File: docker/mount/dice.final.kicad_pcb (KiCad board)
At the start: 2 copper layers, 130 x 130 mm, 303 parts

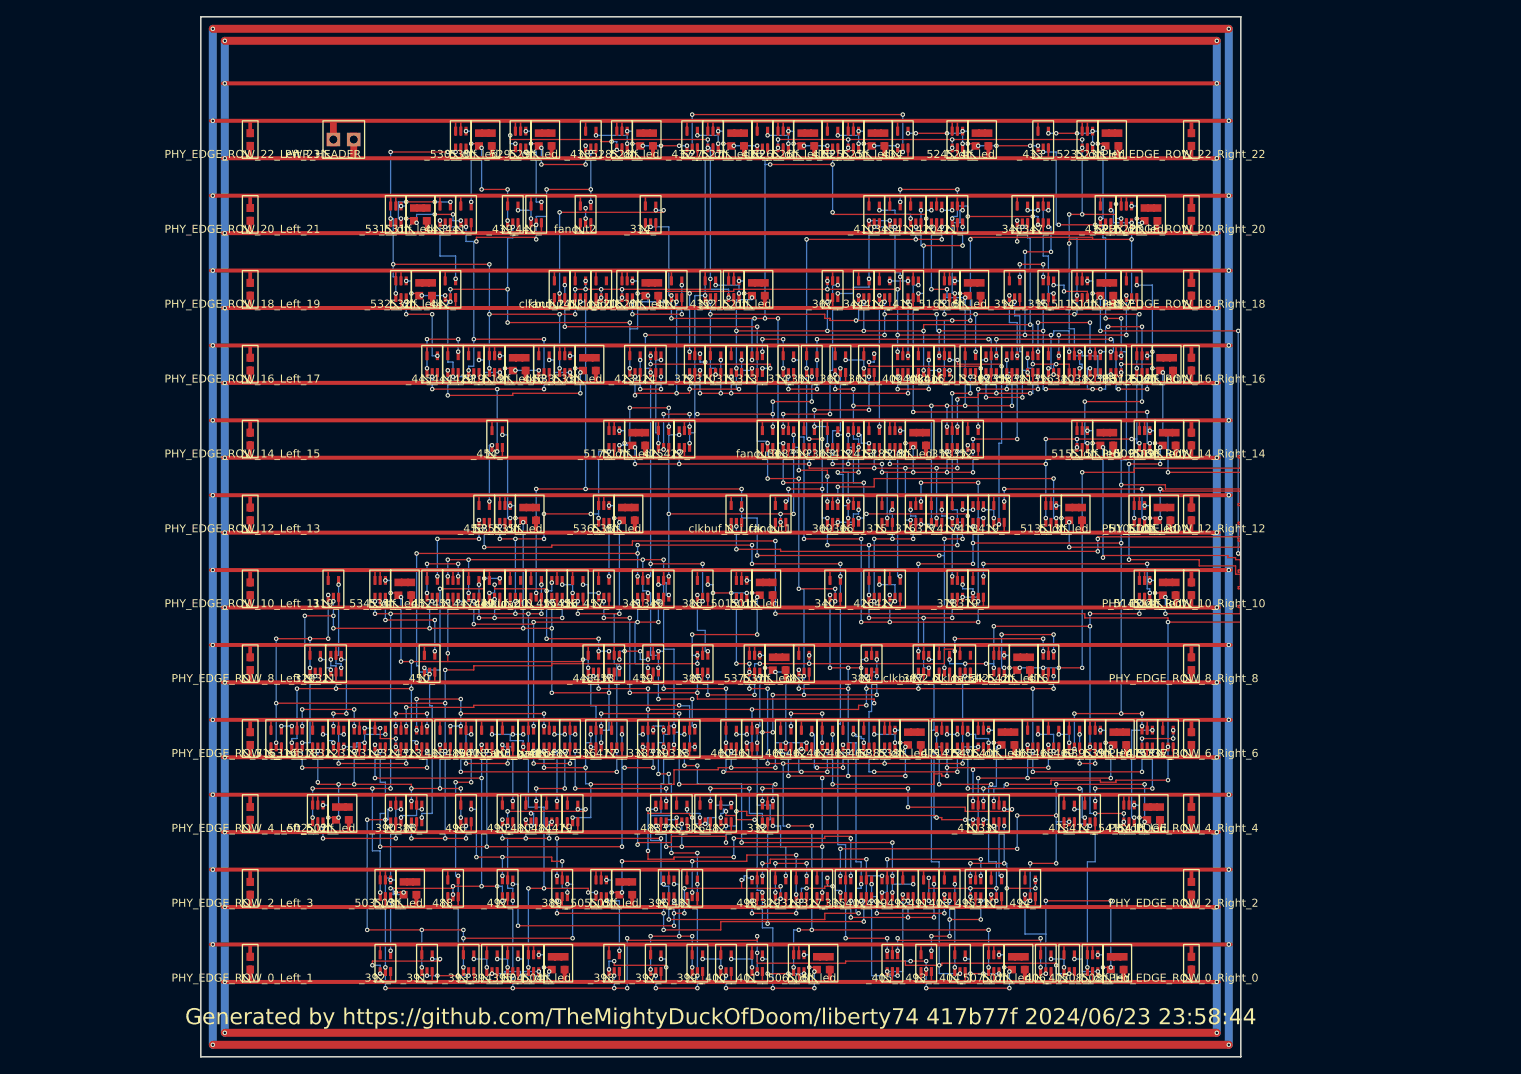
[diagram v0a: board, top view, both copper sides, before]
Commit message: Update example
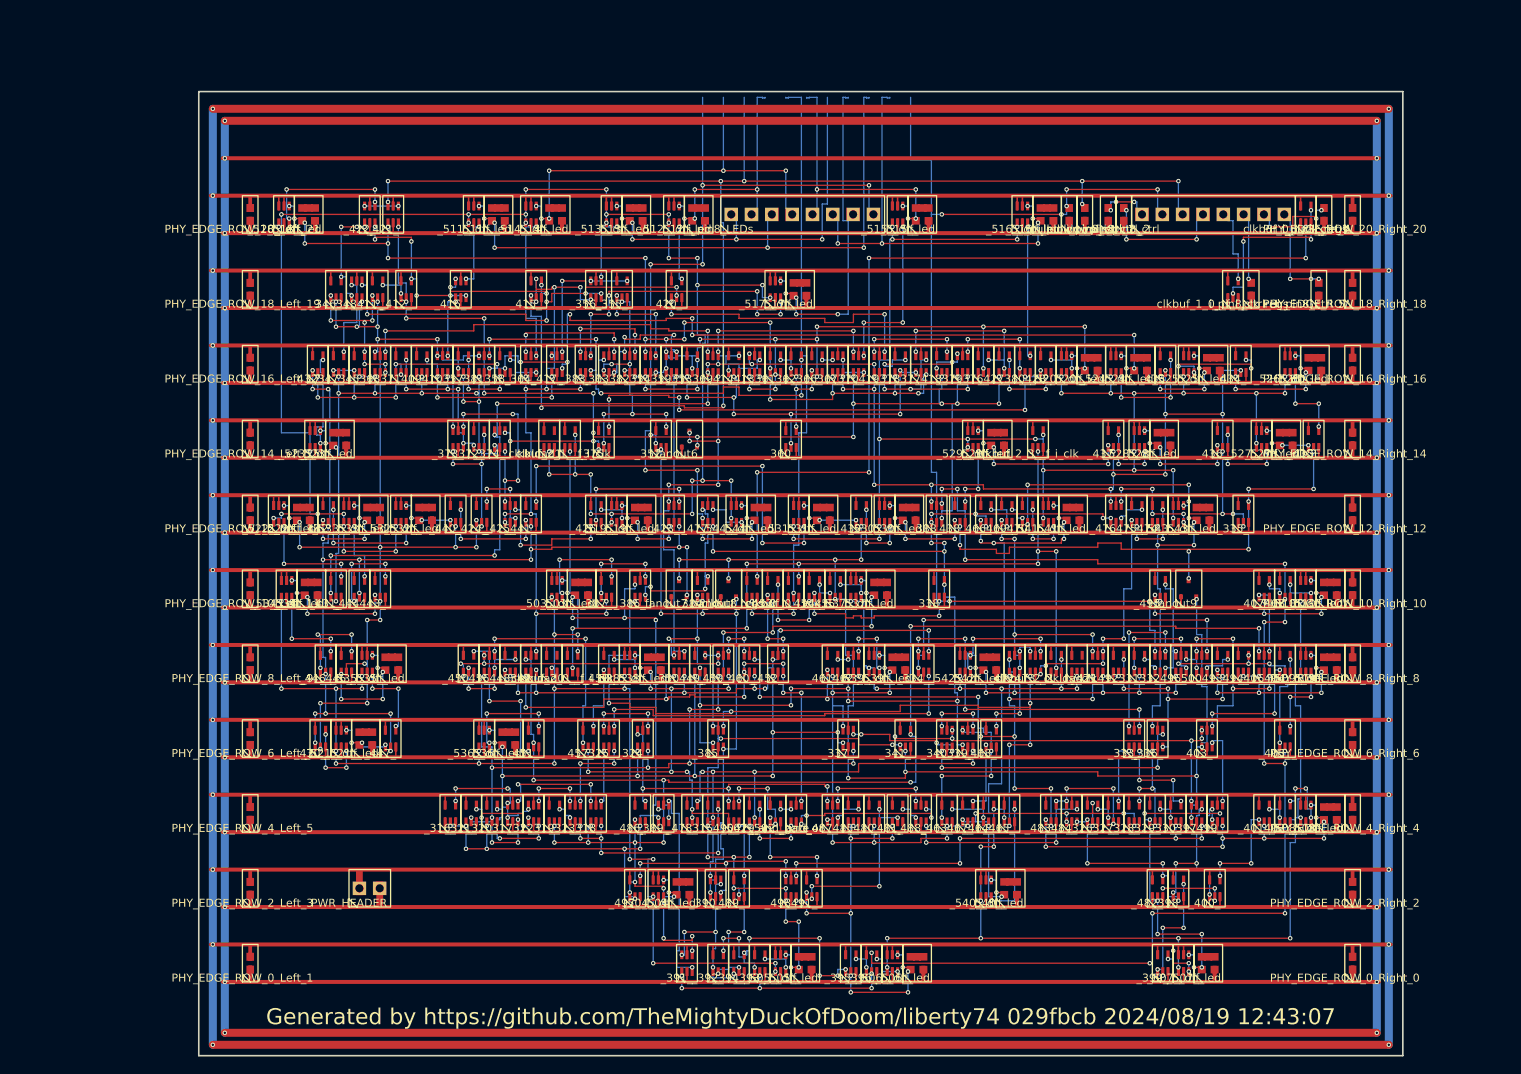
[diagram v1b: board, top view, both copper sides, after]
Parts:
- removed PHY_EDGE_ROW_22_Left_23, PHY_EDGE_ROW_22_Right_22: PWR_CAP, liberty74:PWR_CAP_N
- removed _314_: XOR2_74LVC1G86, liberty74:XOR2_74LVC1G86_N
- removed the _315_ at (8.12, -37.4)
- removed the _316_ at (10.7, -37.4)
- removed the _317_ at (18.5, -37.4)
- removed the _318_ at (13.3, -37.4)
- removed the _319_ at (15.3, -56.2)
- removed the _320_ at (13.0, -46.8)
- removed the _321_ at (15.6, -46.8)
- removed the _322_ at (15.9, -37.4)
- removed the _323_ at (26.3, -37.4)
- removed the _324_ at (23.7, -37.4)
- removed the _325_ at (58.8, -28.1)
- removed the _326_ at (61.8, -28.1)
- removed the _327_ at (76.4, -18.7)
- removed the _328_ at (73.8, -18.7)
- removed the _329_ at (71.2, -18.7)
- removed the _330_ at (98.2, -18.7)
- removed the _331_ at (98.5, -28.1)
- removed the _332_ at (69.5, -28.1)
- removed the _333_ at (59.8, -37.4)
- removed the _334_ at (54.9, -103.0)
- removed the _335_ at (79.3, -18.7)
- removed the _336_ at (48.1, -37.4)
- removed the _337_ at (119.6, -37.4)
- removed the _338_ at (54.6, -37.4)
- removed the _339_ at (57.2, -37.4)
- removed the _340_ at (78.0, -56.2)
- removed the _341_ at (54.0, -56.2)
- removed _344_, _351_: NAND2_74LVC1G00, liberty74:NAND2_74LVC1G00_N
- removed the _346_ at (101.4, -103.0)
- removed the _347_ at (104.0, -103.0)
- removed _349_: NAND3_74LVC1G10, liberty74:NAND3_74LVC1G10_N
- removed the _352_ at (95.2, -74.9)
- removed the _353_ at (100.1, -84.2)
- removed the _354_ at (100.4, -93.6)
- removed the _355_ at (104.7, -93.6)
- removed the _356_ at (105.3, -84.2)
- removed the _357_ at (115.0, -93.6)
- removed the _358_ at (92.6, -74.9)
- removed the _359_ at (74.8, -74.9)
- removed the _360_ at (78.7, -84.2)
- removed the _361_ at (82.2, -84.2)
- removed the _362_ at (97.5, -84.2)
- removed the _363_ at (113.1, -84.2)
- removed _365_, _429_, _500__and_gate: AND2_74LVC1G08, liberty74:AND2_74LVC1G08_N
- removed the _366_ at (80.3, -65.5)
- removed the _367_ at (77.7, -93.6)
- removed the _368_ at (72.2, -74.9)
- removed the _369_ at (77.7, -65.5)
- removed the _370_ at (63.0, -84.2)
- removed the _371_ at (65.7, -84.2)
- removed the _372_ at (60.5, -84.2)
- removed the _373_ at (68.2, -84.2)
- removed the _374_ at (72.2, -84.2)
- removed the _375_ at (84.5, -65.5)
- removed the _376_ at (88.1, -65.5)
- removed the _377_ at (90.7, -65.5)
- removed the _378_ at (93.3, -56.2)
- removed the _379_ at (95.9, -56.2)
- removed the _380_ at (107.9, -84.2)
- removed the _381_ at (102.7, -84.2)
- removed the _382_ at (110.5, -84.2)
- removed the _383_ at (74.1, -46.8)
- removed the _384_ at (82.5, -46.8)
- removed the _385_ at (61.4, -46.8)
- removed the _386_ at (61.4, -56.2)
- removed the _387_ at (89.0, -46.8)
- removed the _389_ at (43.9, -18.7)
- removed the _390_ at (23.1, -28.1)
- removed the _391_ at (27.0, -9.36)
- removed the _392_ at (21.8, -9.36)
- removed the _393_ at (32.2, -9.36)
- removed the _394_ at (35.1, -9.36)
- removed the _395_ at (37.7, -9.36)
- removed the _396_ at (57.2, -18.7)
- removed the _397_ at (55.6, -9.36)
- removed the _398_ at (50.4, -9.36)
- removed the _399_ at (60.8, -9.36)
- removed the _400_ at (64.3, -9.36)
- removed the _401_ at (68.2, -9.36)
- removed the _402_ at (81.9, -18.7)
- removed the _403_ at (92.3, -18.7)
- removed the _404_ at (93.6, -9.36)
- removed the _405_ at (85.2, -9.36)
- removed the _406_ at (104.3, -9.36)
- removed the _407_ at (107.2, -9.36)
- removed the _408_ at (89.0, -84.2)
- removed the _409_ at (86.5, -84.2)
- removed the _410_ at (82.9, -103.0)
- removed the _412_ at (80.3, -74.9)
- removed the _413_ at (82.9, -74.9)
- removed the _414_ at (84.2, -93.6)
- removed the _415_ at (87.8, -93.6)
- removed the _416_ at (91.7, -84.2)
- removed the _417_ at (93.3, -65.5)
- removed the _418_ at (95.9, -65.5)
- removed the _419_ at (98.5, -65.5)
- removed the _420_ at (90.7, -103.0)
- removed the _422_ at (59.1, -74.9)
- removed the _423_ at (53.0, -84.2)
- removed the _424_ at (55.6, -84.2)
- removed the _425_ at (56.5, -74.9)
- removed the _426_ at (82.9, -56.2)
- removed the _427_ at (85.5, -56.2)
- removed the _430_ at (58.2, -93.6)
- removed the _431_ at (62.4, -93.6)
- removed the _432_ at (111.8, -103.0)
- removed the _434_ at (86.5, -112.3)
- removed the _435_ at (77.7, -112.3)
- removed the _437_ at (60.1, -112.3)
- removed the _439_ at (37.7, -103.0)
- removed the _440_ at (40.6, -103.0)
- removed the _442_ at (29.9, -93.6)
- removed the _443_ at (29.2, -103.0)
- removed the _444_ at (30.2, -84.2)
- removed the _445_ at (27.6, -84.2)
- removed the _449_ at (35.4, -56.2)
- removed the _450_ at (27.3, -46.8)
- removed the _451_ at (30.2, -56.2)
- removed the _452_ at (27.6, -56.2)
- removed the _453_ at (34.1, -65.5)
- removed the _454_ at (35.8, -74.9)
- removed the _455_ at (43.2, -56.2)
- removed the _456_ at (45.8, -56.2)
- removed the _457_ at (49.1, -56.2)
- removed the _458_ at (50.4, -46.8)
- removed the _460_ at (65.0, -37.4)
- removed the _461_ at (67.6, -37.4)
- removed the _462_ at (74.4, -37.4)
- removed the _463_ at (79.6, -37.4)
- removed the _464_ at (82.2, -37.4)
- removed the _468_ at (105.3, -37.4)
- removed the _469_ at (107.9, -37.4)
- removed the _470_ at (95.9, -28.1)
- removed the _471_ at (91.3, -37.4)
- removed the _472_ at (93.9, -37.4)
- removed the _473_ at (107.2, -28.1)
- removed the _474_ at (109.8, -28.1)
- removed the _475_ at (117.0, -37.4)
- removed the _477_ at (50.7, -37.4)
- removed the _478_ at (34.5, -37.4)
- removed the _479_ at (45.2, -28.1)
- removed the _480_ at (40.0, -28.1)
- removed the _481_ at (60.1, -18.7)
- removed the _482_ at (64.3, -28.1)
- removed the _483_ at (56.2, -28.1)
- removed the _484_ at (42.6, -28.1)
- removed the _485_ at (29.2, -37.4)
- removed the _486_ at (42.2, -37.4)
- removed the _488_ at (30.2, -18.7)
- removed the _489_ at (31.9, -37.4)
- removed the _490_ at (37.0, -28.1)
- removed the _491_ at (89.7, -18.7)
- removed the _492_ at (87.1, -18.7)
- removed the _493_ at (89.4, -9.36)
- removed the _494_ at (102.4, -18.7)
- removed the _495_ at (95.5, -18.7)
- removed the _496_ at (31.9, -28.1)
- removed the _497_ at (37.0, -18.7)
- removed the _499_ at (84.5, -18.7)
- removed _500__and_or: AO21_74LVC1G0832, liberty74:AO21_74LVC1G0832_N
- removed _501__dff, _502__dff: DFF_74LVC1G175, liberty74:DFF_74LVC1G175_N
- removed _501__led, _502__led: Led_Res_0603, liberty74:Led_Res_0603_N
- removed fanout1, fanout2, fanout3, fanout4: BUF_74LVC1G125, liberty74:BUF_74LVC1G125_N
- added _315_: XOR2_74LVC1G86, liberty74:XOR2_74LVC1G86_N, F.Cu at (62.7, -28.1)
- added _316_: INV_74LVC1G04, liberty74:INV_74LVC1G04_N, F.Cu at (29.9, -28.1)
- added _317_: AND3_74LVC1G11, liberty74:AND3_74LVC1G11_N, F.Cu at (37.7, -28.1)
- added _318_: NAND3_74LVC1G10, liberty74:NAND3_74LVC1G10_N, F.Cu at (48.1, -28.1)
- added _319_: INV_74LVC1G04, liberty74:INV_74LVC1G04_N, F.Cu at (42.9, -28.1)
- added _320_: AND2_74LVC1G08, liberty74:AND2_74LVC1G08_N, F.Cu at (35.1, -28.1)
- added _321_: NOR2_74LVC1G02, liberty74:NOR2_74LVC1G02_N, F.Cu at (32.5, -28.1)
- added _322_: MUX2_74LVC1G157, liberty74:MUX2_74LVC1G157_N, F.Cu at (40.3, -28.1)
- added _323_: NAND3_74LVC1G10, liberty74:NAND3_74LVC1G10_N, F.Cu at (45.5, -28.1)
- added _324_: OR3_74LVC1G332, liberty74:OR3_74LVC1G332_N, F.Cu at (54.0, -37.4)
- added _325_: NAND3_74LVC1G10, liberty74:NAND3_74LVC1G10_N, F.Cu at (49.7, -37.4)
- added _326_: OR2_74LVC1G32, liberty74:OR2_74LVC1G32_N, F.Cu at (110.2, -28.1)
- added _327_: AND2_74LVC1G08, liberty74:AND2_74LVC1G08_N, F.Cu at (112.8, -28.1)
- added _328_: INV_74LVC1G04, liberty74:INV_74LVC1G04_N, F.Cu at (115.4, -28.1)
- added _329_: XOR2_74LVC1G86, liberty74:XOR2_74LVC1G86_N, F.Cu at (118.0, -28.1)
- added _330_: NOR2_74LVC1G02, liberty74:NOR2_74LVC1G02_N, F.Cu at (120.6, -28.1)
- added _331_: OR2_74LVC1G32, liberty74:OR2_74LVC1G32_N, F.Cu at (116.0, -46.8)
- added _332_: AO21_74LVC1G0832, liberty74:AO21_74LVC1G0832_N, F.Cu at (118.6, -46.8)
- added _333_: NOR3_74LVC1G27, liberty74:NOR3_74LVC1G27_N, F.Cu at (115.4, -37.4)
- added _334_: AND3_74LVC1G11, liberty74:AND3_74LVC1G11_N, F.Cu at (89.0, -46.8)
- added _335_: INV_74LVC1G04, liberty74:INV_74LVC1G04_N, F.Cu at (129.0, -65.5)
- added _336_: AND3_74LVC1G11, liberty74:AND3_74LVC1G11_N, F.Cu at (118.3, -37.4)
- added _337_: NOR3_74LVC1G27, liberty74:NOR3_74LVC1G27_N, F.Cu at (79.6, -37.4)
- added _338_: INV_74LVC1G04, liberty74:INV_74LVC1G04_N, F.Cu at (91.0, -56.2)
- added _339_: AND3_74LVC1G11, liberty74:AND3_74LVC1G11_N, F.Cu at (94.6, -37.4)
- added _340_: NAND3_74LVC1G10, liberty74:NAND3_74LVC1G10_N, F.Cu at (92.0, -37.4)
- added _341_: AND2_74LVC1G08, liberty74:AND2_74LVC1G08_N, F.Cu at (86.8, -37.4)
- added _342_: AND3_74LVC1G11, liberty74:AND3_74LVC1G11_N, F.Cu at (40.0, -46.8)
- added _346_: NAND2_74LVC1G00, liberty74:NAND2_74LVC1G00_N, F.Cu at (15.6, -93.6)
- added _347_: OR2_74LVC1G32, liberty74:OR2_74LVC1G32_N, F.Cu at (15.9, -84.2)
- added _348_: MUX2_74LVC1G157, liberty74:MUX2_74LVC1G157_N, F.Cu at (18.2, -93.6)
- added _350_: NAND3_74LVC1G10, liberty74:NAND3_74LVC1G10_N, F.Cu at (58.5, -46.8)
- added _352_: NAND2_74LVC1G00, liberty74:NAND2_74LVC1G00_N, F.Cu at (56.2, -74.9)
- added _353_: NOR2_74LVC1G02, liberty74:NOR2_74LVC1G02_N, F.Cu at (60.1, -84.2)
- added _354_: MUX2_74LVC1G157, liberty74:MUX2_74LVC1G157_N, F.Cu at (54.9, -84.2)
- added _355_: NOR2_74LVC1G02, liberty74:NOR2_74LVC1G02_N, F.Cu at (51.4, -93.6)
- added _356_: AO21_74LVC1G0832, liberty74:AO21_74LVC1G0832_N, F.Cu at (48.1, -93.6)
- added _357_: XOR2_74LVC1G86, liberty74:XOR2_74LVC1G86_N, F.Cu at (31.5, -84.2)
- added _358_: OR2_74LVC1G32, liberty74:OR2_74LVC1G32_N, F.Cu at (36.7, -84.2)
- added _359_: AND3_74LVC1G11, liberty74:AND3_74LVC1G11_N, F.Cu at (57.5, -84.2)
- added _360_: INV_74LVC1G04, liberty74:INV_74LVC1G04_N, F.Cu at (72.5, -74.9)
- added _361_: XOR2_74LVC1G86, liberty74:XOR2_74LVC1G86_N, F.Cu at (70.5, -84.2)
- added _362_: AND2_74LVC1G08, liberty74:AND2_74LVC1G08_N, F.Cu at (73.1, -84.2)
- added _363_: NOR3_74LVC1G27, liberty74:NOR3_74LVC1G27_N, F.Cu at (49.7, -84.2)
- added _364_: AO21_74LVC1G0832, liberty74:AO21_74LVC1G0832_N, F.Cu at (40.0, -84.2)
- added _366_: AND2_74LVC1G08, liberty74:AND2_74LVC1G08_N, F.Cu at (75.7, -84.2)
- added _367_: NOR3_74LVC1G27, liberty74:NOR3_74LVC1G27_N, F.Cu at (78.3, -84.2)
- added _368_: MUX2_74LVC1G157, liberty74:MUX2_74LVC1G157_N, F.Cu at (21.1, -84.2)
- added _369_: NOR3_74LVC1G27, liberty74:NOR3_74LVC1G27_N, F.Cu at (62.7, -84.2)
- added _370_: AO21_74LVC1G0832, liberty74:AO21_74LVC1G0832_N, F.Cu at (80.9, -84.2)
- added _371_: INV_74LVC1G04, liberty74:INV_74LVC1G04_N, F.Cu at (23.7, -84.2)
- added _372_: OR2_74LVC1G32, liberty74:OR2_74LVC1G32_N, F.Cu at (33.5, -74.9)
- added _373_: NAND3_74LVC1G10, liberty74:NAND3_74LVC1G10_N, F.Cu at (30.9, -74.9)
- added _374_: AO21_74LVC1G0832, liberty74:AO21_74LVC1G0832_N, F.Cu at (36.1, -74.9)
- added _375_: AND2_74LVC1G08, liberty74:AND2_74LVC1G08_N, F.Cu at (49.1, -74.9)
- added _376_: INV_74LVC1G04, liberty74:INV_74LVC1G04_N, F.Cu at (96.5, -84.2)
- added _377_: AO21_74LVC1G0832, liberty74:AO21_74LVC1G0832_N, F.Cu at (88.7, -84.2)
- added _378_: OR2_74LVC1G32, liberty74:OR2_74LVC1G32_N, F.Cu at (86.1, -84.2)
- added _379_: AND3_74LVC1G11, liberty74:AND3_74LVC1G11_N, F.Cu at (93.9, -84.2)
- added _380_: NOR2_74LVC1G02, liberty74:NOR2_74LVC1G02_N, F.Cu at (101.7, -84.2)
- added _381_: OR3_74LVC1G332, liberty74:OR3_74LVC1G332_N, F.Cu at (34.1, -84.2)
- added _382_: NOR3_74LVC1G27, liberty74:NOR3_74LVC1G27_N, F.Cu at (52.3, -84.2)
- added _383_: AO21_74LVC1G0832, liberty74:AO21_74LVC1G0832_N, F.Cu at (46.8, -84.2)
- added _384_: NAND2_74LVC1G00, liberty74:NAND2_74LVC1G00_N, F.Cu at (61.4, -56.2)
- added _385_: AND3_74LVC1G11, liberty74:AND3_74LVC1G11_N, F.Cu at (63.4, -37.4)
- added _386_: MUX2_74LVC1G157, liberty74:MUX2_74LVC1G157_N, F.Cu at (53.6, -56.2)
- added _387_: NOR2_74LVC1G02, liberty74:NOR2_74LVC1G02_N, F.Cu at (49.4, -56.2)
- added _389_: AO21_74LVC1G0832, liberty74:AO21_74LVC1G0832_N, F.Cu at (56.5, -28.1)
- added _390_: NAND3_74LVC1G10, liberty74:NAND3_74LVC1G10_N, F.Cu at (63.0, -18.7)
- added _391_: AND3_74LVC1G11, liberty74:AND3_74LVC1G11_N, F.Cu at (59.5, -9.36)
- added _392_: XOR2_74LVC1G86, liberty74:XOR2_74LVC1G86_N, F.Cu at (63.4, -9.36)
- added _393_: AND2_74LVC1G08, liberty74:AND2_74LVC1G08_N, F.Cu at (68.6, -9.36)
- added _394_: NOR2_74LVC1G02, liberty74:NOR2_74LVC1G02_N, F.Cu at (66.0, -9.36)
- added _395_: XOR2_74LVC1G86, liberty74:XOR2_74LVC1G86_N, F.Cu at (80.0, -9.36)
- added _396_: AND2_74LVC1G08, liberty74:AND2_74LVC1G08_N, F.Cu at (82.5, -9.36)
- added _397_: NAND3_74LVC1G10, liberty74:NAND3_74LVC1G10_N, F.Cu at (123.2, -28.1)
- added _398_: XOR2_74LVC1G86, liberty74:XOR2_74LVC1G86_N, F.Cu at (120.9, -18.7)
- added _399_: AND2_74LVC1G08, liberty74:AND2_74LVC1G08_N, F.Cu at (119.0, -9.36)
- added _400_: NOR2_74LVC1G02, liberty74:NOR2_74LVC1G02_N, F.Cu at (125.5, -18.7)
- added _401_: XOR2_74LVC1G86, liberty74:XOR2_74LVC1G86_N, F.Cu at (131.6, -28.1)
- added _402_: AND2_74LVC1G08, liberty74:AND2_74LVC1G08_N, F.Cu at (134.2, -28.1)
- added _403_: NAND3_74LVC1G10, liberty74:NAND3_74LVC1G10_N, F.Cu at (124.5, -37.4)
- added _404_: XOR2_74LVC1G86, liberty74:XOR2_74LVC1G86_N, F.Cu at (134.2, -46.8)
- added _405_: AND2_74LVC1G08, liberty74:AND2_74LVC1G08_N, F.Cu at (134.2, -37.4)
- added _406_: AND3_74LVC1G11, liberty74:AND3_74LVC1G11_N, F.Cu at (131.6, -46.8)
- added _407_: XOR2_74LVC1G86, liberty74:XOR2_74LVC1G86_N, F.Cu at (131.6, -56.2)
- added _408_: AND2_74LVC1G08, liberty74:AND2_74LVC1G08_N, F.Cu at (134.2, -56.2)
- added _409_: INV_74LVC1G04, liberty74:INV_74LVC1G04_N, F.Cu at (26.3, -84.2)
- added _410_: NAND3_74LVC1G10, liberty74:NAND3_74LVC1G10_N, F.Cu at (28.9, -84.2)
- added _412_: NOR2_74LVC1G02, liberty74:NOR2_74LVC1G02_N, F.Cu at (24.4, -93.6)
- added _413_: NOR3_74LVC1G27, liberty74:NOR3_74LVC1G27_N, F.Cu at (67.9, -84.2)
- added _414_: AND2_74LVC1G08, liberty74:AND2_74LVC1G08_N, F.Cu at (65.3, -84.2)
- added _415_: NOR2_74LVC1G02, liberty74:NOR2_74LVC1G02_N, F.Cu at (40.6, -93.6)
- added _416_: AO21_74LVC1G0832, liberty74:AO21_74LVC1G0832_N, F.Cu at (31.2, -93.6)
- added _417_: NAND3_74LVC1G10, liberty74:NAND3_74LVC1G10_N, F.Cu at (43.2, -84.2)
- added _418_: NAND2_74LVC1G00, liberty74:NAND2_74LVC1G00_N, F.Cu at (91.3, -84.2)
- added _419_: OR3_74LVC1G332, liberty74:OR3_74LVC1G332_N, F.Cu at (83.5, -84.2)
- added _420_: AND2_74LVC1G08, liberty74:AND2_74LVC1G08_N, F.Cu at (58.2, -93.6)
- added _422_: AO21_74LVC1G0832, liberty74:AO21_74LVC1G0832_N, F.Cu at (19.8, -103.0)
- added _423_: AND3_74LVC1G11, liberty74:AND3_74LVC1G11_N, F.Cu at (57.9, -65.5)
- added _424_: OR2_74LVC1G32, liberty74:OR2_74LVC1G32_N, F.Cu at (33.8, -65.5)
- added _425_: AND3_74LVC1G11, liberty74:AND3_74LVC1G11_N, F.Cu at (37.4, -65.5)
- added _426_: OR2_74LVC1G32, liberty74:OR2_74LVC1G32_N, F.Cu at (48.1, -65.5)
- added _427_: AND2_74LVC1G08, liberty74:AND2_74LVC1G08_N, F.Cu at (99.1, -84.2)
- added _428_: NOR2_74LVC1G02, liberty74:NOR2_74LVC1G02_N, F.Cu at (104.3, -84.2)
- added _430_: AND2_74LVC1G08, liberty74:AND2_74LVC1G08_N, F.Cu at (13.7, -37.4)
- added _431_: OR2_74LVC1G32, liberty74:OR2_74LVC1G32_N, F.Cu at (15.6, -56.2)
- added _432_: AND2_74LVC1G08, liberty74:AND2_74LVC1G08_N, F.Cu at (13.3, -84.2)
- added _434_: OR2_74LVC1G32, liberty74:OR2_74LVC1G32_N, F.Cu at (128.7, -84.2)
- added _435_: AND2_74LVC1G08, liberty74:AND2_74LVC1G08_N, F.Cu at (137.8, -74.9)
- added _437_: OR2_74LVC1G32, liberty74:OR2_74LVC1G32_N, F.Cu at (112.8, -74.9)
- added _439_: AND2_74LVC1G08, liberty74:AND2_74LVC1G08_N, F.Cu at (81.2, -65.5)
- added _440_: XOR2_74LVC1G86, liberty74:XOR2_74LVC1G86_N, F.Cu at (30.6, -65.5)
- added _442_: AND2_74LVC1G08, liberty74:AND2_74LVC1G08_N, F.Cu at (14.6, -65.5)
- added _443_: XOR2_74LVC1G86, liberty74:XOR2_74LVC1G86_N, F.Cu at (21.1, -56.2)
- added _444_: AND2_74LVC1G08, liberty74:AND2_74LVC1G08_N, F.Cu at (18.5, -56.2)
- added _445_: XOR2_74LVC1G86, liberty74:XOR2_74LVC1G86_N, F.Cu at (16.9, -46.8)
- added _449_: AND2_74LVC1G08, liberty74:AND2_74LVC1G08_N, F.Cu at (61.1, -46.8)
- added _450_: XOR2_74LVC1G86, liberty74:XOR2_74LVC1G86_N, F.Cu at (32.2, -46.8)
- added _451_: AND2_74LVC1G08, liberty74:AND2_74LVC1G08_N, F.Cu at (40.3, -37.4)
- added _452_: AND3_74LVC1G11, liberty74:AND3_74LVC1G11_N, F.Cu at (70.8, -46.8)
- added _453_: XOR2_74LVC1G86, liberty74:XOR2_74LVC1G86_N, F.Cu at (70.2, -56.2)
- added _454_: OR2_74LVC1G32, liberty74:OR2_74LVC1G32_N, F.Cu at (75.4, -56.2)
- added _455_: AND2_74LVC1G08, liberty74:AND2_74LVC1G08_N, F.Cu at (78.0, -56.2)
- added _456_: AND3_74LVC1G11, liberty74:AND3_74LVC1G11_N, F.Cu at (34.8, -46.8)
- added _457_: XOR2_74LVC1G86, liberty74:XOR2_74LVC1G86_N, F.Cu at (47.1, -37.4)
- added _458_: AND2_74LVC1G08, liberty74:AND2_74LVC1G08_N, F.Cu at (49.7, -46.8)
- added _460_: AND3_74LVC1G11, liberty74:AND3_74LVC1G11_N, F.Cu at (67.3, -46.8)
- added _461_: XOR2_74LVC1G86, liberty74:XOR2_74LVC1G86_N, F.Cu at (77.7, -46.8)
- added _462_: AND3_74LVC1G11, liberty74:AND3_74LVC1G11_N, F.Cu at (80.3, -46.8)
- added _463_: AND2_74LVC1G08, liberty74:AND2_74LVC1G08_N, F.Cu at (92.0, -28.1)
- added _464_: XOR2_74LVC1G86, liberty74:XOR2_74LVC1G86_N, F.Cu at (97.2, -28.1)
- added _468_: AND2_74LVC1G08, liberty74:AND2_74LVC1G08_N, F.Cu at (97.5, -37.4)
- added _469_: XOR2_74LVC1G86, liberty74:XOR2_74LVC1G86_N, F.Cu at (99.5, -65.5)
- added _470_: OR2_74LVC1G32, liberty74:OR2_74LVC1G32_N, F.Cu at (102.0, -65.5)
- added _471_: NAND3_74LVC1G10, liberty74:NAND3_74LVC1G10_N, F.Cu at (110.8, -46.8)
- added _472_: AO21_74LVC1G0832, liberty74:AO21_74LVC1G0832_N, F.Cu at (100.4, -46.8)
- added _473_: AND3_74LVC1G11, liberty74:AND3_74LVC1G11_N, F.Cu at (103.0, -46.8)
- added _474_: INV_74LVC1G04, liberty74:INV_74LVC1G04_N, F.Cu at (118.3, -65.5)
- added _475_: XOR2_74LVC1G86, liberty74:XOR2_74LVC1G86_N, F.Cu at (115.7, -65.5)
- added _477_: AO21_74LVC1G0832, liberty74:AO21_74LVC1G0832_N, F.Cu at (62.1, -65.5)
- added _478_: INV_74LVC1G04, liberty74:INV_74LVC1G04_N, F.Cu at (60.1, -28.1)
- added _479_: AND2_74LVC1G08, liberty74:AND2_74LVC1G08_N, F.Cu at (67.9, -28.1)
- added _480_: INV_74LVC1G04, liberty74:INV_74LVC1G04_N, F.Cu at (82.9, -28.1)
- added _481_: AND2_74LVC1G08, liberty74:AND2_74LVC1G08_N, F.Cu at (85.8, -28.1)
- added _482_: INV_74LVC1G04, liberty74:INV_74LVC1G04_N, F.Cu at (118.3, -18.7)
- added _483_: XOR2_74LVC1G86, liberty74:XOR2_74LVC1G86_N, F.Cu at (105.0, -28.1)
- added _484_: AO21_74LVC1G0832, liberty74:AO21_74LVC1G0832_N, F.Cu at (107.6, -28.1)
- added _485_: INV_74LVC1G04, liberty74:INV_74LVC1G04_N, F.Cu at (80.3, -28.1)
- added _486_: NAND2_74LVC1G00, liberty74:NAND2_74LVC1G00_N, F.Cu at (53.6, -28.1)
- added _488_: AO21_74LVC1G0832, liberty74:AO21_74LVC1G0832_N, F.Cu at (88.7, -28.1)
- added _489_: INV_74LVC1G04, liberty74:INV_74LVC1G04_N, F.Cu at (66.0, -18.7)
- added _490_: AO21_74LVC1G0832, liberty74:AO21_74LVC1G0832_N, F.Cu at (65.3, -28.1)
- added _491_: XOR2_74LVC1G86, liberty74:XOR2_74LVC1G86_N, F.Cu at (75.1, -18.7)
- added _492_: INV_74LVC1G04, liberty74:INV_74LVC1G04_N, F.Cu at (113.4, -46.8)
- added _493_: XOR2_74LVC1G86, liberty74:XOR2_74LVC1G86_N, F.Cu at (126.4, -46.8)
- added _494_: INV_74LVC1G04, liberty74:INV_74LVC1G04_N, F.Cu at (129.0, -46.8)
- added _495_: XOR2_74LVC1G86, liberty74:XOR2_74LVC1G86_N, F.Cu at (118.6, -56.2)
- added _496_: AO21_74LVC1G0832, liberty74:AO21_74LVC1G0832_N, F.Cu at (121.2, -46.8)
- added _497_: AND2_74LVC1G08, liberty74:AND2_74LVC1G08_N, F.Cu at (53.0, -18.7)
- added _499_: AND3_74LVC1G11, liberty74:AND3_74LVC1G11_N, F.Cu at (125.8, -28.1)
- added _500_: MUX2_74LVC1G157, liberty74:MUX2_74LVC1G157_N, F.Cu at (123.8, -46.8)
- added _502__and_gate: AND2_74LVC1G08, liberty74:AND2_74LVC1G08_N, F.Cu at (70.5, -28.1)
- added _502__and_or: AO21_74LVC1G0832, liberty74:AO21_74LVC1G0832_N, F.Cu at (73.1, -28.1)
- added _543__dff: DFF_74LVC1G175, liberty74:DFF_74LVC1G175_N, F.Cu at (120.9, -65.5)
- added _543__led: Led_Res_0603, liberty74:Led_Res_0603_N, F.Cu at (123.5, -65.5)
- added _544__dff: DFF_74LVC1G175, liberty74:DFF_74LVC1G175_N, F.Cu at (65.7, -65.5)
- added _544__led: Led_Res_0603, liberty74:Led_Res_0603_N, F.Cu at (68.2, -65.5)
- added clkbuf_0_i_clk_regs: BUF_74LVC1G125, liberty74:BUF_74LVC1G125_N, F.Cu at (136.8, -103.0)
- added clkbuf_1_0__f_i_clk_regs: BUF_74LVC1G125, liberty74:BUF_74LVC1G125_N, F.Cu at (127.7, -93.6)
- added clkbuf_regs_0_: BUF_74LVC1G125, liberty74:BUF_74LVC1G125_N, F.Cu at (67.6, -56.2)
- added fanout6: DS9809PRSS3, liberty74:DS9809PRSS3_N, F.Cu at (59.5, -74.9)
- added fanout7: DS9809PRSS3, liberty74:DS9809PRSS3_N, F.Cu at (58.2, -56.2)
- added fanout8: DS9809PRSS3, liberty74:DS9809PRSS3_N, F.Cu at (64.3, -56.2)
- added fanout9: DS9809PRSS3, liberty74:DS9809PRSS3_N, F.Cu at (121.9, -56.2)
- added i_pin8_LEDs: PINOUT_8, liberty74:PINOUT_8_N, F.Cu at (65.0, -103.0)
- added i_pin8_ctrl: PINOUT_8, liberty74:PINOUT_8_N, F.Cu at (116.3, -103.0)
- added i_pin8_ctrl_1: TIE_LO, liberty74:TIE_LO_N, F.Cu at (112.5, -103.0)
- added i_pin8_ctrl_2: TIE_LO, liberty74:TIE_LO_N, F.Cu at (114.4, -103.0)
- added i_pin8_ctrl_3: TIE_LO, liberty74:TIE_LO_N, F.Cu at (130.3, -93.6)
- added i_pin8_ctrl_4: TIE_LO, liberty74:TIE_LO_N, F.Cu at (139.4, -103.0)
- added i_pin8_ctrl_5: TIE_LO, liberty74:TIE_LO_N, F.Cu at (138.8, -93.6)
- added i_pulldown_roll: PULLDOWN_R0603, liberty74:PULLDOWN_R0603_N, F.Cu at (107.6, -103.0)
- added i_pulldown_rst: PULLDOWN_R0603, liberty74:PULLDOWN_R0603_N, F.Cu at (109.5, -103.0)
- moved _522__dff 112.4 mm to (8.45, -65.5)
- moved _522__led 112.4 mm to (11.1, -65.5)
- moved _523__dff 103.5 mm to (13.0, -74.9)
- moved _523__led 103.5 mm to (15.6, -74.9)
- moved PWR_HEADER 93.7 mm to (18.5, -18.7)
- moved _514__dff 89.9 mm to (40.0, -103.0)
- moved _514__led 89.9 mm to (42.6, -103.0)
- moved _518__dff 81.4 mm to (9.10, -103.0)
- moved _518__led 81.4 mm to (11.7, -103.0)
- moved _527__dff 78.1 mm to (131.3, -74.9)
- moved _527__led 78.1 mm to (133.9, -74.9)
- moved _511__dff 76.6 mm to (32.8, -103.0)
- moved _511__led 76.6 mm to (35.4, -103.0)
- moved _388_ 75.0 mm to (90.7, -65.5)
- moved _528__dff 74.7 mm to (116.0, -74.9)
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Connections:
- net bcd[0] renamed segments\[5\]
- net bcd[1] renamed segments\[6\]
- net clkdiv[1] renamed lfsr\[14\]
- net clkdiv[2] renamed clkdiv\[0\]
- net counter[2] renamed counter\[0\]
- net counter[3] renamed counter\[1\]
- net counter[4] renamed counter\[2\]
- net counter[5] renamed counter\[3\]
- net counter[6] renamed counter\[4\]
- net counter[7] renamed counter\[5\]
- net lfsr[13] renamed lfsr\[11\]
- net lfsr[14] renamed lfsr\[12\]
- net lfsr[7] renamed lfsr\[5\]
- net segments[0] renamed segments\[2\]
- net segments[1] renamed counter\[7\]
- net segments[2] renamed counter\[6\]
- net segments[3] renamed segments\[1\]
- net segments[4] renamed segments\[0\]
- net segments[5] renamed segments\[3\]
- net segments[6] renamed segments\[4\]
- _345_ pad 1: _077_ -> lfsr\[3\]
- _345_ pad 2: lfsr[1] -> lfsr\[2\]
- _345_ pad 4: _078_ -> _077_
- _388_ pad 1: counter[0] -> _070_
- _388_ pad 3: _073_ -> net6
- _388_ pad 4: _115_ -> _114_
- _388_ pad 6: counter[1] -> RST
- _411_ pad 1: _130_ -> _077_
- _411_ pad 2: net1 -> lfsr\[1\]
- _411_ pad 4: _131_ -> _130_
- _421_ pad 1: _078_ -> bcd\[0\]
- _421_ pad 3: _131_ -> net6
- _421_ pad 4: _015_ -> _138_
- _421_ pad 6: _138_ -> RST
- _433_ pad 1: lfsr[5] -> lfsr\[4\]
- _433_ pad 4: _022_ -> _021_
- _436_ pad 1: lfsr[8] -> lfsr\[7\]
- _436_ pad 4: _025_ -> _024_
- _438_ pad 1: lfsr[10] -> lfsr\[9\]
- _438_ pad 2: net2 -> _067_
- _438_ pad 4: _027_ -> _026_
- _441_ pad 1: lfsr[12] -> _144_
- _441_ pad 2: net2 -> net7
- _441_ pad 4: _029_ -> _028_
- _446_ pad 1: lfsr[0] -> _146_
- _446_ pad 2: net2 -> net7
- _446_ pad 4: _032_ -> _031_
- _447_ pad 1: _066_ -> lfsr\[0\]
- _447_ pad 2: _183_ -> net7
- _447_ pad 4: _147_ -> _032_
- _448_ pad 1: clkdiv[0] -> _066_
- _448_ pad 2: _070_ -> _183_
- _448_ pad 4: _148_ -> _147_
- _459_ pad 1: _183_ -> clkdiv\[1\]
- _459_ pad 3: _066_ -> clkdiv\[2\]
- _459_ pad 4: _156_ -> _155_
- _459_ pad 6: _155_ -> _148_
- _465_ pad 1: clkdiv[5] -> _159_
- _465_ pad 2: _070_ -> _112_
- _465_ pad 4: _160_ -> _037_
- _466_ pad 1: clkdiv[4] -> clkdiv\[5\]
- _466_ pad 2: clkdiv[3] -> _070_
- _466_ pad 4: _161_ -> _160_
- _467_ pad 1: _161_ -> clkdiv\[4\]
- _467_ pad 2: _156_ -> clkdiv\[3\]
- _467_ pad 4: _162_ -> _161_
- _476_ pad 1: dp -> _070_
- _476_ pad 3: _070_ -> _167_
- _476_ pad 4: _041_ -> _040_
- _476_ pad 6: _111_ -> RST
- _487_ pad 1: _171_ -> clkdiv\[3\]
- _487_ pad 3: _174_ -> _175_
- _487_ pad 4: _178_ -> _177_
- _487_ pad 6: _177_ -> _176_
- _498_ pad 4: _045_ -> _044_
- _498_ pad 6: _044_ -> _043_
- _503__dff pad 3: _007_ -> _005_
- _504__dff pad 3: _008_ -> _006_
- _505__dff pad 3: _009_ -> _007_
- _506__dff pad 3: _010_ -> _008_
- _507__dff pad 3: _011_ -> _009_
- _508__dff pad 3: _012_ -> _010_
- _509__dff pad 1: clknet_2_3__leaf_i_clk -> clknet_2_2__leaf_i_clk
- _509__dff pad 3: _013_ -> _011_
- _510__dff pad 1: clknet_2_3__leaf_i_clk -> clknet_2_2__leaf_i_clk
- _510__dff pad 3: _014_ -> _012_
- _511__dff pad 1: clknet_2_3__leaf_i_clk -> clknet_2_1__leaf_i_clk
- _511__dff pad 3: _000_ -> _013_
- _512__dff pad 1: clknet_2_3__leaf_i_clk -> clknet_2_1__leaf_i_clk
- _512__dff pad 3: _001_ -> _014_
- _513__dff pad 1: clknet_2_3__leaf_i_clk -> clknet_2_1__leaf_i_clk
- _513__dff pad 3: _002_ -> _000_
- _514__dff pad 1: clknet_2_2__leaf_i_clk -> clknet_2_1__leaf_i_clk
- _514__dff pad 3: _003_ -> _001_
- _515__dff pad 3: _004_ -> _002_
- _516__dff pad 3: _015_ -> _003_
- _517__dff pad 1: clknet_2_0__leaf_i_clk -> clknet_2_1__leaf_i_clk
- _517__dff pad 3: _016_ -> _004_
- _518__dff pad 1: clknet_2_3__leaf_i_clk -> clknet_2_1__leaf_i_clk
- _518__dff pad 3: _017_ -> _015_
- _518__dff pad 4: bcd[2] -> bcd\[0\]
- _518__led pad 1: bcd[2] -> bcd\[0\]
- _519__dff pad 3: _018_ -> _016_
- _519__dff pad 4: lfsr[0] -> bcd\[1\]
- _519__led pad 1: lfsr[0] -> bcd\[1\]
- _520__dff pad 1: clknet_2_1__leaf_i_clk -> clknet_2_3__leaf_i_clk
- _520__dff pad 3: _019_ -> _017_
- _520__dff pad 4: lfsr[1] -> bcd\[2\]
- _520__led pad 1: lfsr[1] -> bcd\[2\]
- _521__dff pad 1: clknet_2_1__leaf_i_clk -> clknet_2_0__leaf_i_clk
- _521__dff pad 3: _020_ -> _018_
- _521__dff pad 4: lfsr[2] -> lfsr\[0\]
- _521__led pad 1: lfsr[2] -> lfsr\[0\]
- _522__dff pad 1: clknet_2_3__leaf_i_clk -> clknet_2_1__leaf_i_clk
- _522__dff pad 3: _021_ -> _019_
- _522__dff pad 4: lfsr[3] -> lfsr\[1\]
- _522__led pad 1: lfsr[3] -> lfsr\[1\]
- _523__dff pad 1: clknet_2_3__leaf_i_clk -> clknet_2_1__leaf_i_clk
- _523__dff pad 3: _022_ -> _020_
- _523__dff pad 4: lfsr[4] -> lfsr\[2\]
- _523__led pad 1: lfsr[4] -> lfsr\[2\]
- _524__dff pad 3: _023_ -> _021_
- _524__dff pad 4: lfsr[5] -> lfsr\[3\]
- _524__led pad 1: lfsr[5] -> lfsr\[3\]
- _525__dff pad 3: _024_ -> _022_
- _525__dff pad 4: lfsr[6] -> lfsr\[4\]
- _525__led pad 1: lfsr[6] -> lfsr\[4\]
- _526__dff pad 3: _025_ -> _023_
- _527__dff pad 1: clknet_2_1__leaf_i_clk -> clknet_2_3__leaf_i_clk
- _527__dff pad 3: _026_ -> _024_
- _527__dff pad 4: lfsr[8] -> lfsr\[6\]
- _527__led pad 1: lfsr[8] -> lfsr\[6\]
- _528__dff pad 1: clknet_2_1__leaf_i_clk -> clknet_2_3__leaf_i_clk
- _528__dff pad 3: _027_ -> _025_
- _528__dff pad 4: lfsr[9] -> lfsr\[7\]
- _528__led pad 1: lfsr[9] -> lfsr\[7\]
- _529__dff pad 1: clknet_2_1__leaf_i_clk -> clknet_2_3__leaf_i_clk
- _529__dff pad 3: _028_ -> _026_
- _529__dff pad 4: lfsr[10] -> lfsr\[8\]
- _529__led pad 1: lfsr[10] -> lfsr\[8\]
- _530__dff pad 1: clknet_2_1__leaf_i_clk -> clknet_2_3__leaf_i_clk
- _530__dff pad 3: _029_ -> _027_
- _530__dff pad 4: lfsr[11] -> lfsr\[9\]
- _530__led pad 1: lfsr[11] -> lfsr\[9\]
- _531__dff pad 1: clknet_2_1__leaf_i_clk -> clknet_2_3__leaf_i_clk
- _531__dff pad 3: _030_ -> _028_
- _531__dff pad 4: lfsr[12] -> lfsr\[10\]
- _531__led pad 1: lfsr[12] -> lfsr\[10\]
- _532__dff pad 3: _031_ -> _029_
- _533__dff pad 3: _032_ -> _030_
- _534__dff pad 3: _033_ -> _031_
- _534__dff pad 4: clkdiv[0] -> lfsr\[13\]
- _534__led pad 1: clkdiv[0] -> lfsr\[13\]
- _535__dff pad 3: _034_ -> _032_
- _536__dff pad 3: _035_ -> _033_
- _537__dff pad 3: _036_ -> _034_
- _537__dff pad 4: clkdiv[3] -> clkdiv\[1\]
- _537__led pad 1: clkdiv[3] -> clkdiv\[1\]
- _538__dff pad 1: clknet_2_2__leaf_i_clk -> clknet_2_0__leaf_i_clk
- _538__dff pad 3: _037_ -> _035_
- _538__dff pad 4: clkdiv[4] -> clkdiv\[2\]
- _538__led pad 1: clkdiv[4] -> clkdiv\[2\]
- _539__dff pad 3: _038_ -> _036_
- _539__dff pad 4: clkdiv[5] -> clkdiv\[3\]
- _539__led pad 1: clkdiv[5] -> clkdiv\[3\]
- _540__dff pad 3: _039_ -> _037_
- _540__dff pad 4: clkdiv[6] -> clkdiv\[4\]
- _540__led pad 1: clkdiv[6] -> clkdiv\[4\]
- _541__dff pad 1: clknet_2_2__leaf_i_clk -> clknet_2_3__leaf_i_clk
- _541__dff pad 3: _040_ -> _038_
- _541__dff pad 4: clkdiv[7] -> clkdiv\[5\]
- _541__led pad 1: clkdiv[7] -> clkdiv\[5\]
- _542__dff pad 3: _041_ -> _039_
- _542__dff pad 4: dp -> clkdiv\[6\]
- _542__led pad 1: dp -> clkdiv\[6\]
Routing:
- net net4: track 182.8 -> 9.88 mm, vias 25 -> 3
- net lfsr[1]: track 171.2 -> 0.00 mm, vias 30 -> 0
- net net9: track 0.00 -> 140.5 mm, vias 0 -> 16
- net net6: track 0.00 -> 138.9 mm, vias 0 -> 21
- net lfsr\[1\]: track 0.00 -> 138.4 mm, vias 0 -> 29
- net lfsr\[3\]: track 0.00 -> 138.1 mm, vias 0 -> 21
- net GND: track 2114.5 -> 2250.0 mm, vias 30 -> 28
- net counter[0]: track 133.0 -> 0.00 mm, vias 22 -> 0
- net clkdiv\[1\]: track 0.00 -> 131.3 mm, vias 0 -> 22
- net net7: track 0.00 -> 126.4 mm, vias 0 -> 20
- net lfsr[3]: track 123.3 -> 0.00 mm, vias 18 -> 0
- net lfsr[2]: track 120.6 -> 0.00 mm, vias 23 -> 0
- net bcd\[0\]: track 0.00 -> 120.6 mm, vias 0 -> 24
- net VDD: track 2038.0 -> 2150.5 mm, vias 28 -> 26
- net i_clk_regs: track 0.00 -> 112.3 mm, vias 0 -> 6
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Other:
- board size 130 x 130 mm -> 150.5 x 120.5 mm
- rule pad_to_mask_clearance: 0.0 -> 0
- board text added: "Generated by https://github.com/TheMightyDuckOfDoom/liberty74 029fbcb 2024/08/19 12:43:07"
- board text removed: "Generated by https://github.com/TheMightyDuckOfDoom/liberty74 417b77f 2024/06/23 23:58:44"
